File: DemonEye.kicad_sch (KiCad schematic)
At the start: 50 parts, among them CN1 PicoBlade 1x07 P1.25mm, Q1 CSD25501F3, Q2 CSD25501F3, Q3 CSD25501F3, Q4 CSD25501F3, Q5 CSD25501F3, U1 WS2814F, U2 LMZM23601

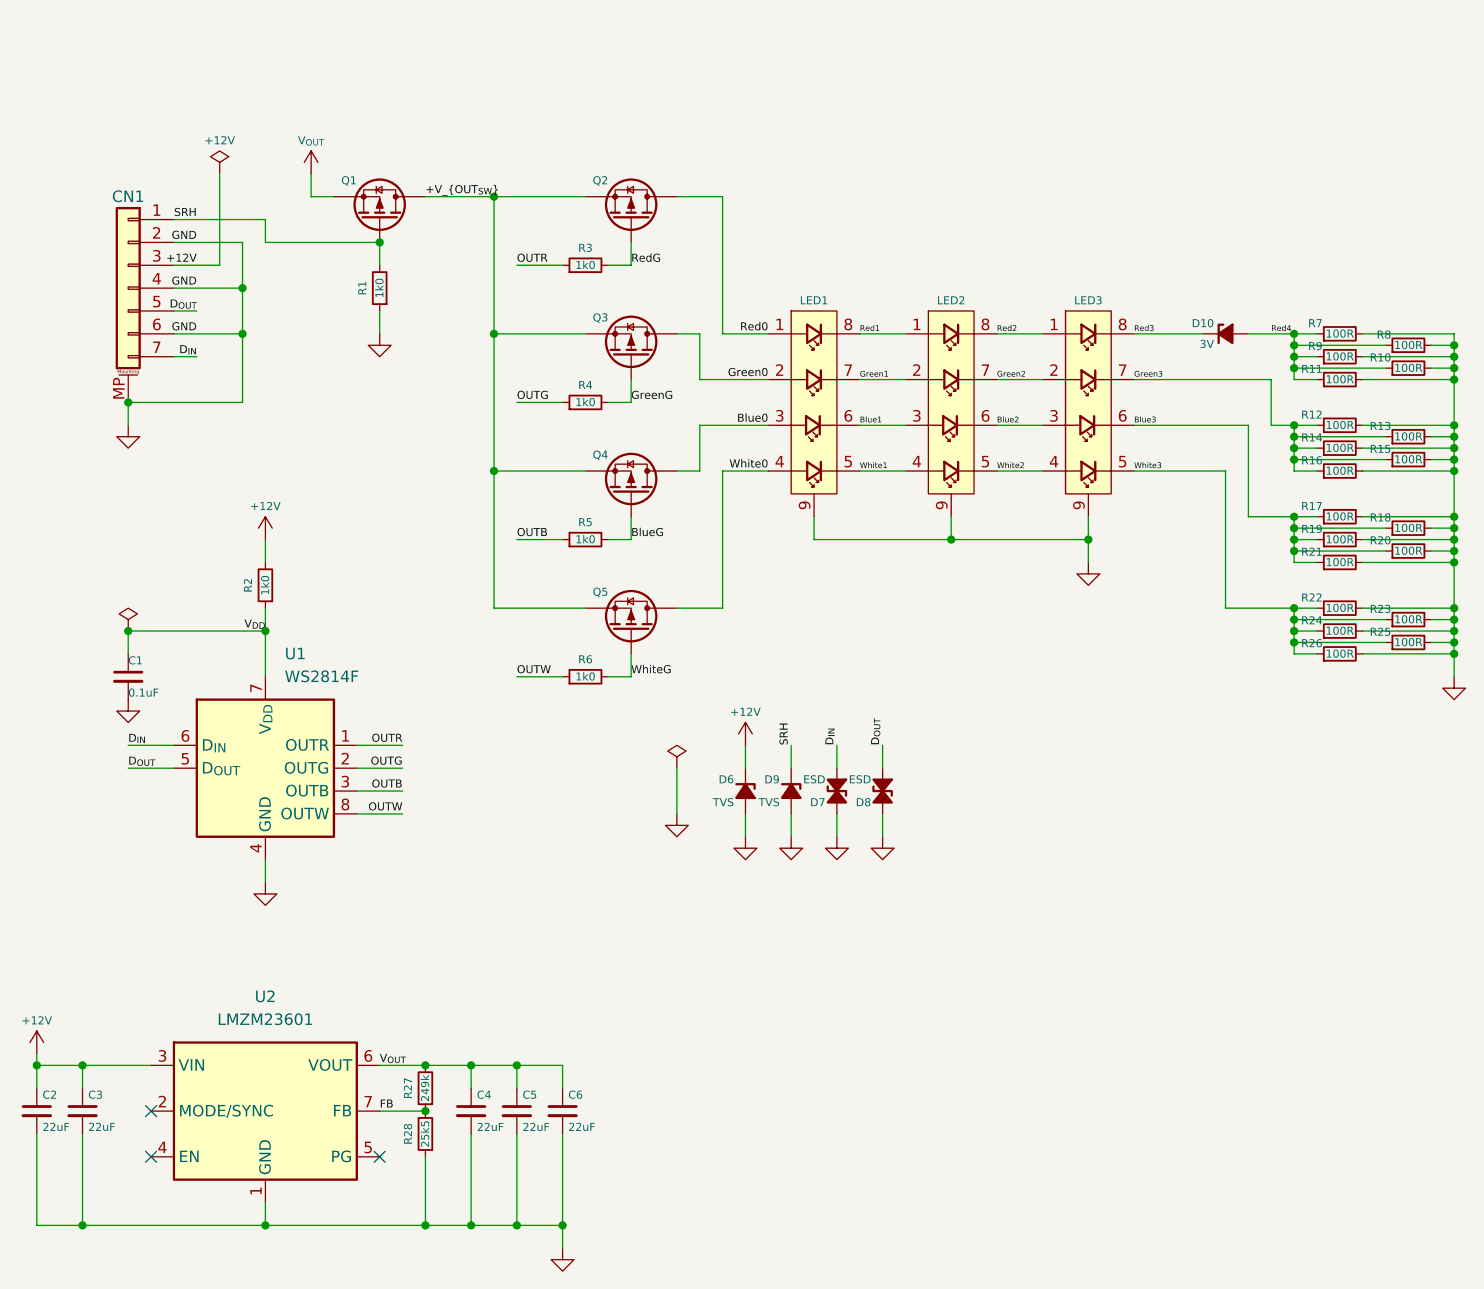
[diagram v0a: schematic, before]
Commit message: v0.4.0.0
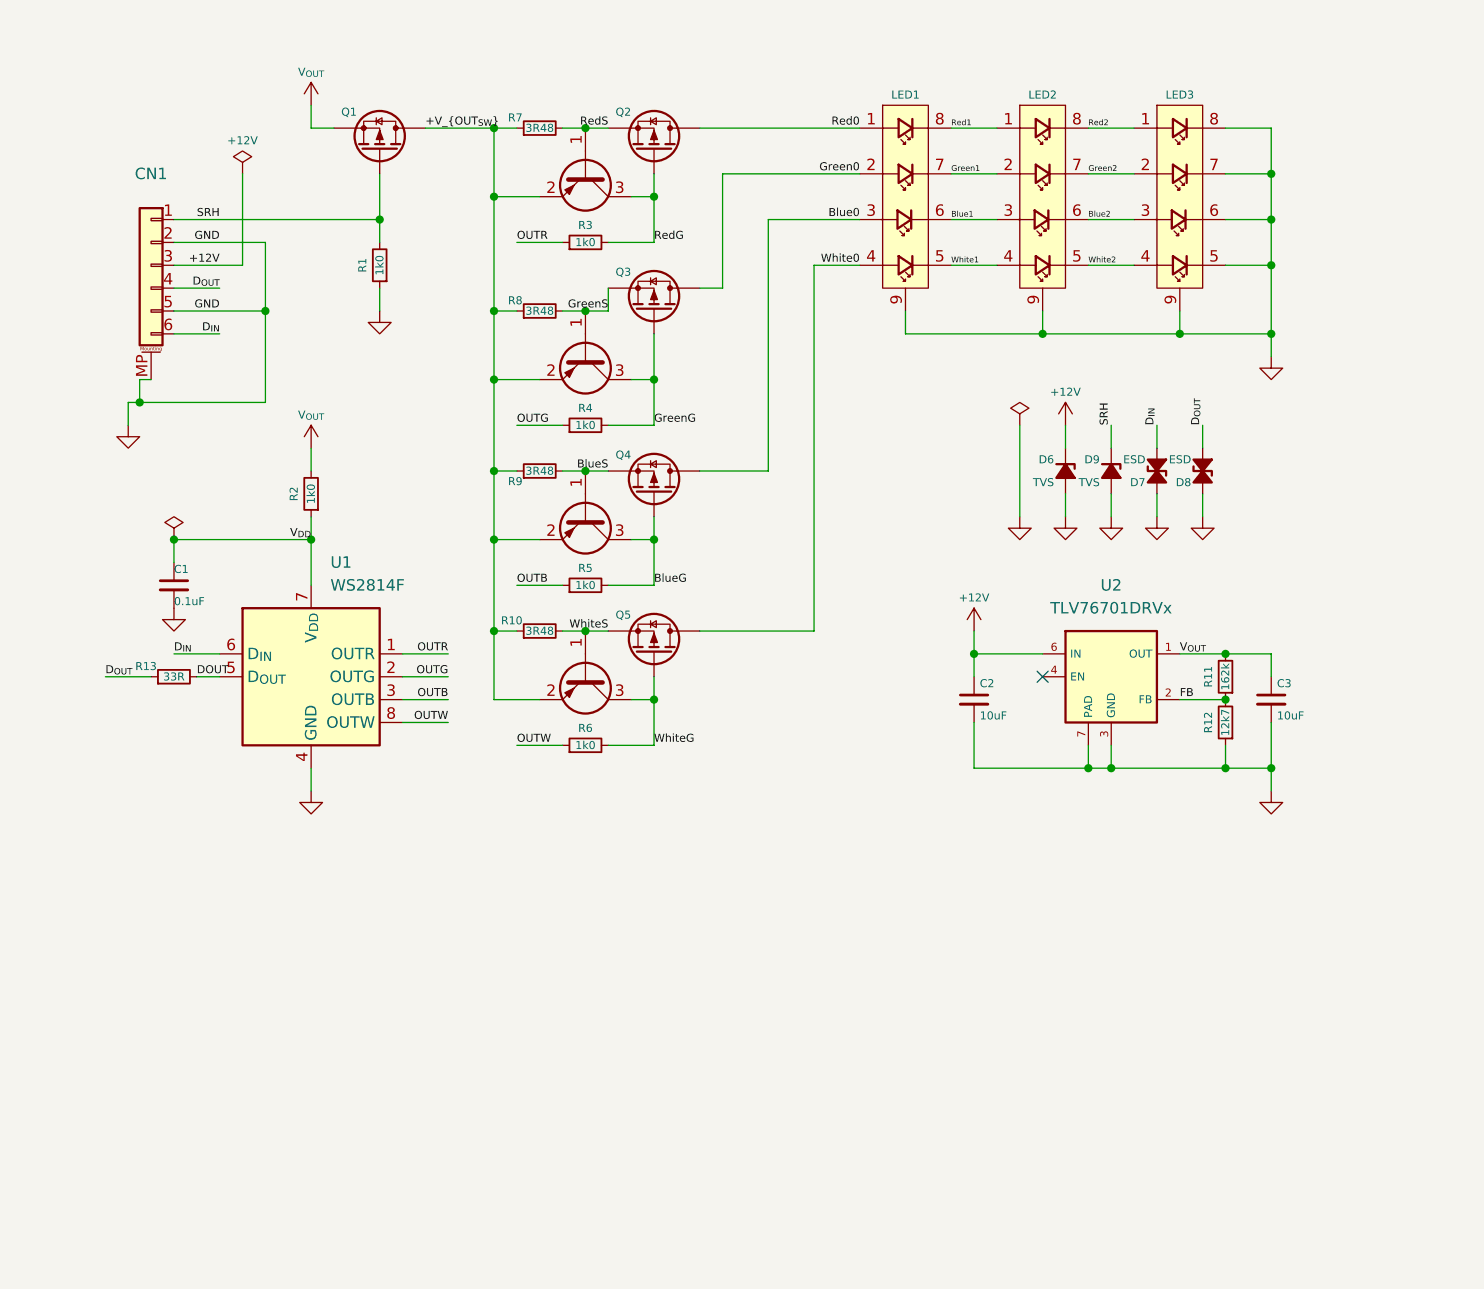
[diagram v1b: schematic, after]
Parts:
- removed C4, C5, C6: 22uF, My Capacitors:C_0603_Dense, symbol Device:C_Small
- removed D10: 3V, My Package_Leadless:DFN1006-2, symbol PersonalSchematicSymbolLibrary:D_Zener_Small_Filled
- removed R11, R12, R14, R15, R16, R17, R18, R19, R20, R21, R22, R23, R24, R25, R26: 100R, My Resistors:R_0201_Dense, symbol Device:R_Small
- removed U2: LMZM23601, My Package_Leadless:Texas_SIL0010A_MicroSiP-10-1EP_3.8x3mm_P0.6mm_EP0.7x2.9mm, symbol Regulator_Switching:LMZM23601
- added Q10, Q6, Q8, Q9: BC807-25QAZ, My Package_Leadless:DFN1010D-3, symbol Transistor_BJT:Q_PNP_BEC
- added U2: TLV76701DRVx, My Package_Leadless:WSON-6-1EP_2x2mm_P0.65mm_EP1x1.6mm, symbol My Power Management:TLV76701DRVx
- C2, C3: value 22uF -> 10uF; Distributor Link 1 https://www.digikey.com/en/products/detail/murata-electronics/GRM188C61E226ME01D/22528498 -> https://www.digikey.com/en/products/detail/murata-electronics/GRM188R6YA106MA73D/5877411; Distributor Link 2 https://www.mouser.com/ProductDetail/Murata-Electronics/GRM188C61E226ME01D?qs=Z%252BL2brAPG1JcH41Chu2%252B6A%3D%3D -> https://www.mouser.com/ProductDetail/Murata-Electronics/GRM188R6YA106MA73D?qs=I53XXhTNm8uKsiF7Obn3Gg%3D%3D; LCSC C29519229 -> C194427; Manufacturer Part Number GRM188C61E226ME01D -> GRM188R6YA106MA73D
- CN1: footprint My Connectors:Molex_PicoBlade_53261-0771_1x07_P1.25mm_Horizontal_SMD -> My Connectors:Molex_PicoBlade_53261-0671_1x06_P1.25mm_Horizontal_SMD; symbol PersonalSchematicSymbolLibrary:Conn_01x07_MountingPin -> PersonalSchematicSymbolLibrary:Conn_01x06_MountingPin
- R10, R7, R8, R9: value 100R -> 3R48; footprint My Resistors:R_0201_Dense -> My Resistors:R_0402_Nominal; Distributor Link 1 https://www.digikey.com/en/products/detail/yageo/AC0201FR-0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 -> https://www.digikey.com/en/products/detail/yageo/AC0402FR-0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; Distributor Link 2 https://www.mouser.com/ProductDetail/YAGEO/AC0201FR-07100RL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 -> https://www.mouser.com/ProductDetail/YAGEO/AC0402FR-073R48L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; LCSC C226395 -> C227058; Manufacturer Part Number AC0201FR-07100RL -> AC0402FR-073R48L
- R11: renamed from R27; value 249k -> 162k; Distributor Link 1 https://www.digikey.com/en/products/detail/yageo/RC0201FR-0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 -> (none); Distributor Link 2 https://www.mouser.com/ProductDetail/YAGEO/RC0201FR-07249KL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 -> (none); LCSC C273273 -> C320713; Manufacturer YAGEO -> FH (Guangdong Fenghua Advanced Tech); Manufacturer Part Number RC0201FR-07249KL -> RC-01W1623FT
- R12: renamed from R28; value 25k5 -> 12k7; Distributor Link 1 https://www.digikey.com/en/products/detail/yageo/AC0201FR-0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 -> (none); Distributor Link 2 https://www.mouser.com/ProductDetail/YAGEO/AC0201FR-0725K5L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 -> https://www.mouser.com/ProductDetail/Royalohm/0201WMF1272TE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; LCSC C910623 -> C423755; Manufacturer YAGEO -> UNI-ROYAL(Uniroyal Elec); Manufacturer Part Number AC0201FR-0725K5L -> 0201WMF1272TEE
- R13: value 100R -> 33R; footprint My Resistors:R_0201_Dense -> My Resistors:R_0201_Nominal; Distributor Link 1 https://www.digikey.com/en/products/detail/yageo/AC0201FR-07100RL/5894218 -> https://www.digikey.com/en/products/detail/yageo/AC0201FR-0733RL/5894558; Distributor Link 2 https://www.mouser.com/ProductDetail/YAGEO/AC0201FR-07100RL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 -> https://www.mouser.com/ProductDetail/YAGEO/AC0201FR-0733RL?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; LCSC C226395 -> C226514; Manufacturer Part Number AC0201FR-07100RL -> AC0201FR-0733RL
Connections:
- net Blue3 is gone; now on net GND: LED3.6 (Blue_K)
- net Red3 is gone; now on net GND: LED3.8 (Red_K)
- net Red4 is gone; now on net +V_{OUT_{SW}}: R10.1, R7.1, R8.1, R9.1
- net White3 is gone; now on net GND: LED3.5 (White_K)
- net +12V: now also U2.6 (IN); no longer C3.1, R2.2
- net +V_{OUT_{SW}}: now also Q10.2 (E), Q6.2 (E), Q8.2 (E), Q9.2 (E); no longer Q2.2 (S), Q3.2 (S), Q4.2 (S), Q5.2 (S)
- net BlueG: now also Q9.3 (C)
- net D_{IN}: now also CN1.6 (Pin_4); no longer CN1.7 (Pin_5)
- net D_{OUT}: now also CN1.4 (Pin_4), R13.1; no longer CN1.5 (Pin_5), U1.5 (D_{OUT})
- net FB: now also U2.2 (FB)
- net GND: now also CN1.5 (Pin_4), LED3.7 (Green_K), U2.3 (GND), U2.5 (GND), U2.7 (PAD); no longer CN1.4 (Pin_4), CN1.6 (Pin_5), R10.2, R13.2, R7.2, R8.2, R9.2
- net GreenG: now also Q8.3 (C)
- net RedG: now also Q6.3 (C)
- net V_{OUT}: now also C3.1, R2.2, U2.1 (OUT)
- net WhiteG: now also Q10.3 (C)
- removed net Green3: LED3.7 (Green_K), R13.1
- new net BlueS: Q4.2 (S), Q9.1 (B), R9.2
- new net DOUT: R13.2, U1.5 (D_{OUT})
- new net GreenS: Q3.2 (S), Q8.1 (B), R8.2
- new net RedS: Q2.2 (S), Q6.1 (B), R7.2
- new net WhiteS: Q10.1 (B), Q5.2 (S), R10.2
- no-connect marks 3 -> 1
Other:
- moved on the sheet: C1, C2, C3, D6, D7, D8, D9, LED1, LED2, LED3, Q1, Q2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

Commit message: Update ConstantCurrentWithThermalFoldbackDesign.txt, DemonEye.kicad_pcb, DemonEye.kicad_prl, and 3 more files
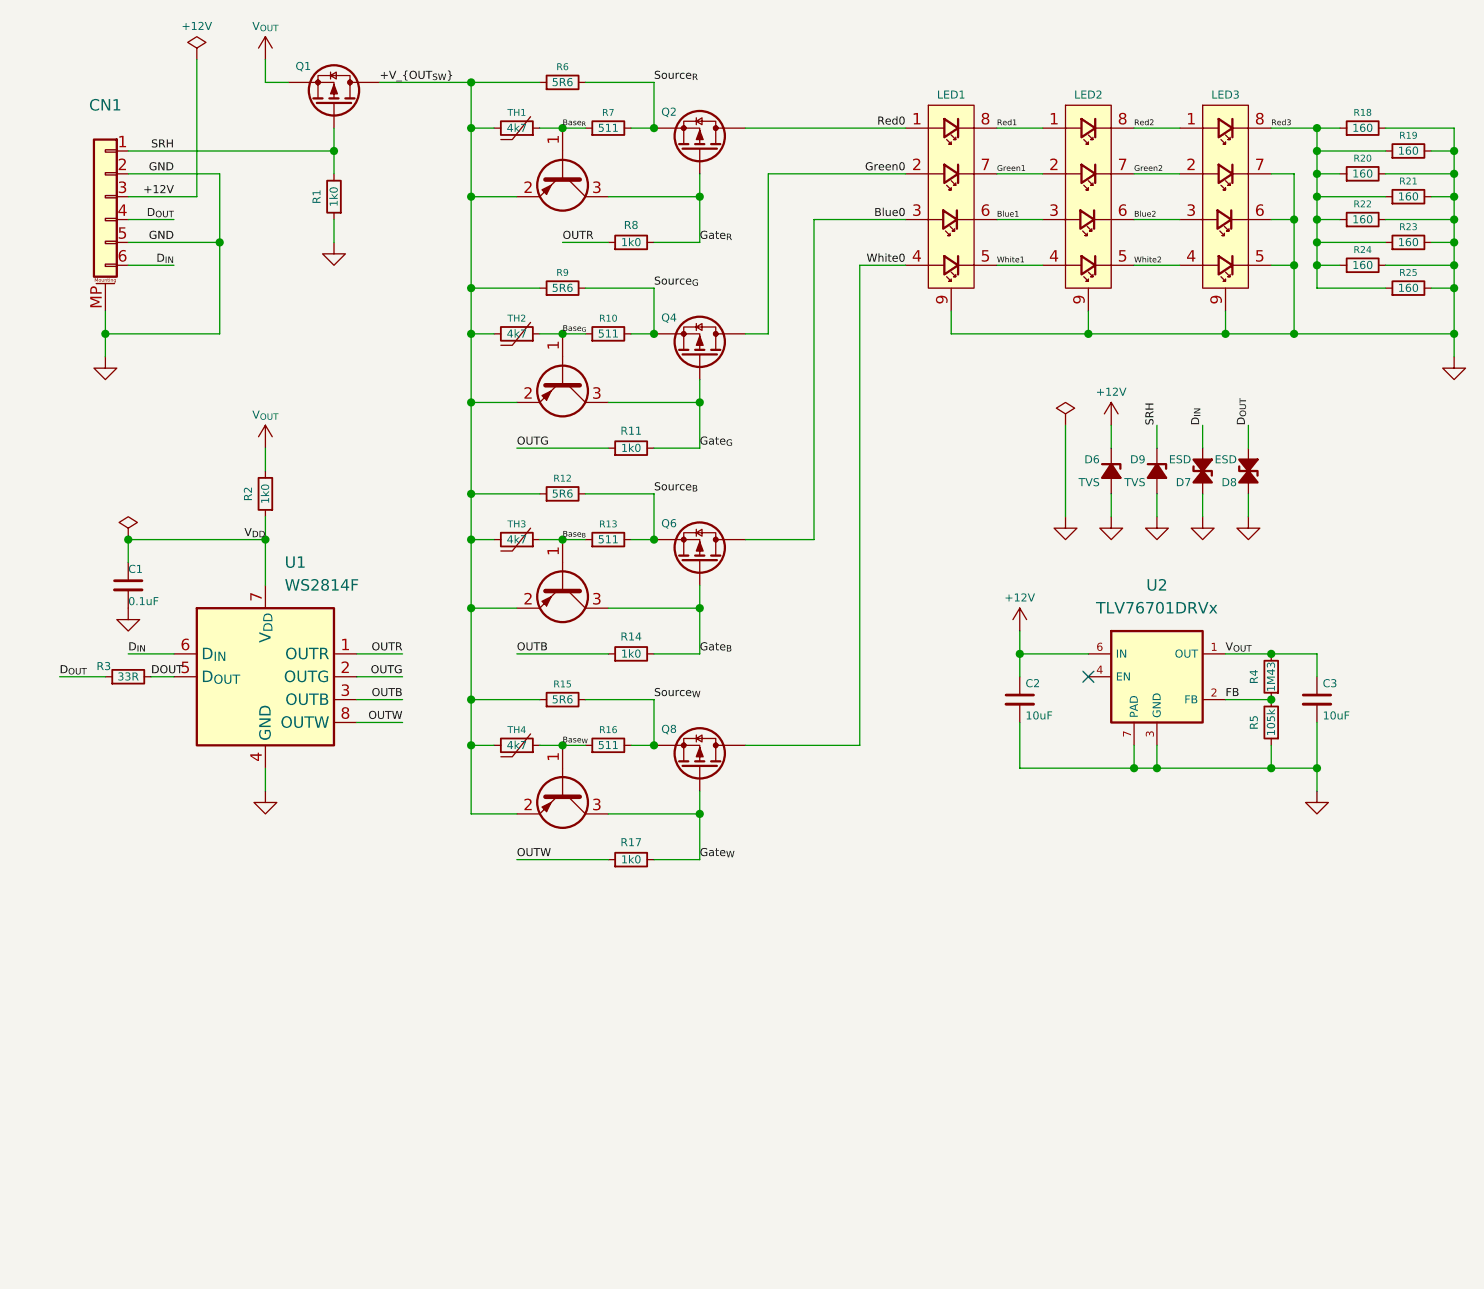
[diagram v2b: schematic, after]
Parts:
- removed R4, R5, R6: 1k0, My Resistors:R_0402_Nominal, symbol Device:R_Small
- removed R8: 3R48, My Resistors:R_0402_Nominal, symbol Device:R_Small
- added R11, R14, R17: 1k0, My Resistors:R_0402_Nominal, symbol Device:R_Small
- added R12, R15: 5R6, My Resistors:R_0402_Nominal, symbol Device:R_Small
- added R13, R16, R7: 511, My Resistors:R_0201_Dense, symbol Device:R_Small
- added R18, R19, R20, R21, R22, R23, R24, R25: 160, My Resistors:R_0201_Dense, symbol Device:R_Small
- added TH1, TH2, TH3, TH4: 4k7, My Resistors:TH_0402_Nominal, symbol PersonalSchematicSymbolLibrary:TH_Small
- CN1: value PicoBlade 1x07 P1.25mm -> PicoBlade 1x06 P1.25mm; Distributor Link 1 https://www.digikey.com/en/products/detail/molex/0532610771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 -> https://www.digikey.com/en/products/detail/molex/0532610671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; Distributor Link 2 https://www.mouser.com/ProductDetail/Molex/53261-0771?qs=%2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 -> https://www.mouser.com/ProductDetail/Molex/53261-0671?qs=%2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; LCSC C2845384 -> C2845383; Manufacturer Part Number HC-1.25-7PWT -> HC-1.25-6PWT
- R10: value 3R48 -> 511; footprint My Resistors:R_0402_Nominal -> My Resistors:R_0201_Dense; Distributor Link 1 https://www.digikey.com/en/products/detail/yageo/AC0402FR-0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 -> https://www.digikey.com/en/products/detail/walsin-technolog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; Distributor Link 2 https://www.mouser.com/ProductDetail/YAGEO/AC0402FR-073R48L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 -> https://www.mouser.com/ProductDetail/Walsin/WR02X5110FAL?qs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; LCSC C227058 -> C367646; Manufacturer YAGEO -> Walsin Tech Corp; Manufacturer Part Number AC0402FR-073R48L -> WR02X5110FAL
- R4: renamed from R11; value 162k -> 1M43; footprint My Resistors:R_0201_Nominal -> My Resistors:R_0201_Dense; Distributor Link 2 (none) -> https://www.mouser.com/ProductDetail/Royalohm/0201WMF1434TE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; LCSC C320713 -> C784121; Manufacturer FH (Guangdong Fenghua Advanced Tech) -> UNI-ROYAL(Uniroyal Elec); Manufacturer Part Number RC-01W1623FT -> (none)
- R5: renamed from R12; value 12k7 -> 105k; footprint My Resistors:R_0201_Nominal -> My Resistors:R_0201_Dense; Distributor Link 1 (none) -> https://www.digikey.com/en/products/detail/yageo/AC0201FR-0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; Distributor Link 2 https://www.mouser.com/ProductDetail/Royalohm/0201WMF1272TE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 -> https://www.mouser.com/ProductDetail/YAGEO/AC0201FR-07105KL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; LCSC C423755 -> C226397; Manufacturer UNI-ROYAL(Uniroyal Elec) -> YAGEO; Manufacturer Part Number 0201WMF1272TEE -> AC0201FR-07105KL
- R6: renamed from R7; value 3R48 -> 5R6; Distributor Link 1 https://www.digikey.com/en/products/detail/yageo/AC0402FR-0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 -> https://www.digikey.com/en/products/detail/koa-speer-electr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; Distributor Link 2 https://www.mouser.com/ProductDetail/YAGEO/AC0402FR-073R48L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 -> https://www.mouser.com/ProductDetail/KOA-Speer/RK73H1ETTP5R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; LCSC C227058 -> C830259; Manufacturer YAGEO -> KOA Speer Elec; Manufacturer Part Number AC0402FR-073R48L -> RK73H1ETTP5R60F
- R9: value 3R48 -> 5R6; Distributor Link 1 https://www.digikey.com/en/products/detail/yageo/AC0402FR-0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 -> https://www.digikey.com/en/products/detail/koa-speer-electr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; Distributor Link 2 https://www.mouser.com/ProductDetail/YAGEO/AC0402FR-073R48L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 -> https://www.mouser.com/ProductDetail/KOA-Speer/RK73H1ETTP5R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; LCSC C227058 -> C830259; Manufacturer YAGEO -> KOA Speer Elec; Manufacturer Part Number AC0402FR-073R48L -> RK73H1ETTP5R60F
- renumbered Q6 to Q3, Q3 to Q4, Q8 to Q5, Q4 to Q6, Q9 to Q7, Q5 to Q8, Q10 to Q9, R13 to R3, R3 to R8
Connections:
- net +V_{OUT_{SW}}: now also R12.1, R15.1, TH1.2, TH2.2, TH3.2, TH4.2; no longer R10.1
- net GND: now also R18.2, R19.2, R20.2, R21.2, R22.2, R23.2, R24.2, R25.2; no longer LED3.8 (Red_K)
- net OUTB: now also R14.1
- net OUTG: now also R11.1
- net OUTW: now also R17.1
- net BlueG renamed Gate_{B}
- net Gate_{B}: now also R14.2
- removed net BlueS: Q6.2 (S), Q7.1 (B), R9.2
- net GreenG renamed Gate_{G}
- net Gate_{G}: now also R11.2
- net GreenS renamed Base_{G}
- net Base_{G}: now also R10.1, TH2.1; no longer Q4.2 (S)
- net RedG renamed Gate_{R}
- net RedS renamed Source_{R}
- net Source_{R}: now also R7.2; no longer Q3.1 (B)
- net WhiteG renamed Gate_{W}
- net Gate_{W}: now also R17.2
- removed net WhiteS: Q8.2 (S), Q9.1 (B), R10.2
- new net Base_{B}: Q7.1 (B), R13.1, TH3.1
- new net Base_{R}: Q3.1 (B), R7.1, TH1.1
- new net Base_{W}: Q9.1 (B), R16.1, TH4.1
- new net Red3: LED3.8 (Red_K), R18.1, R19.1, R20.1, R21.1, R22.1, R23.1, R24.1, R25.1
- new net Source_{B}: Q6.2 (S), R12.2, R13.2
- new net Source_{G}: Q4.2 (S), R10.2, R9.2
- new net Source_{W}: Q8.2 (S), R15.2, R16.2
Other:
- moved on the sheet: C1, C2, C3, CN1, D6, D7, D8, D9, LED1, LED2, LED3, Q1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
